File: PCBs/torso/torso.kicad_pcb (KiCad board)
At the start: 4 copper layers, 140 x 81 mm, 84 parts, among them J3 USB_B_Micro, Q1_RLY_CTRL1 Q_NIGBT_CGE, SW1 RESET, U1 TJA1057GT/3J, U2 LM317_TO-220, U3 LM317_TO-220, U4 STM32F303RETx

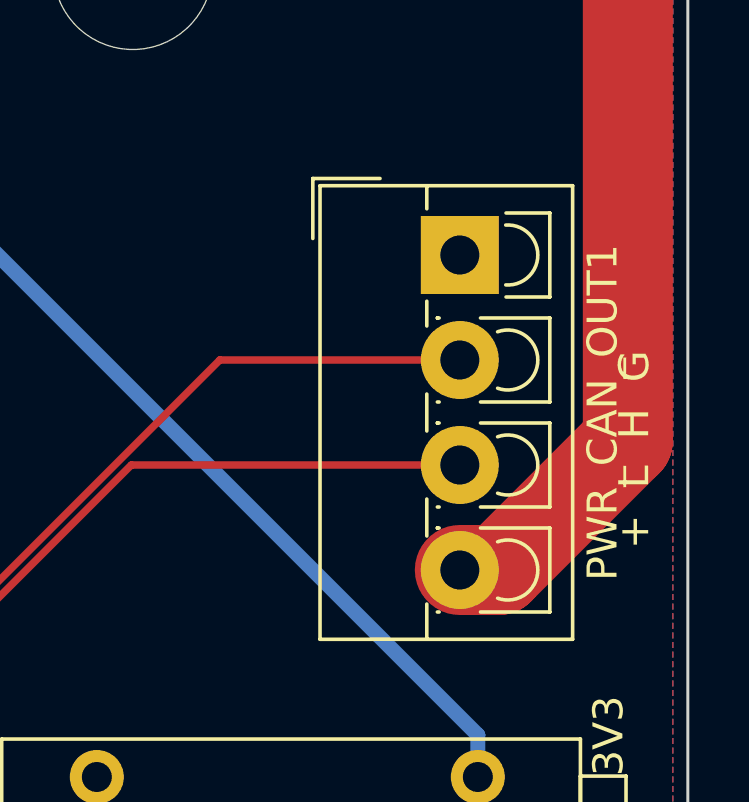
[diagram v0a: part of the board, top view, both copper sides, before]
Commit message: All revisions finished, MK1.1 ready for gerber generation
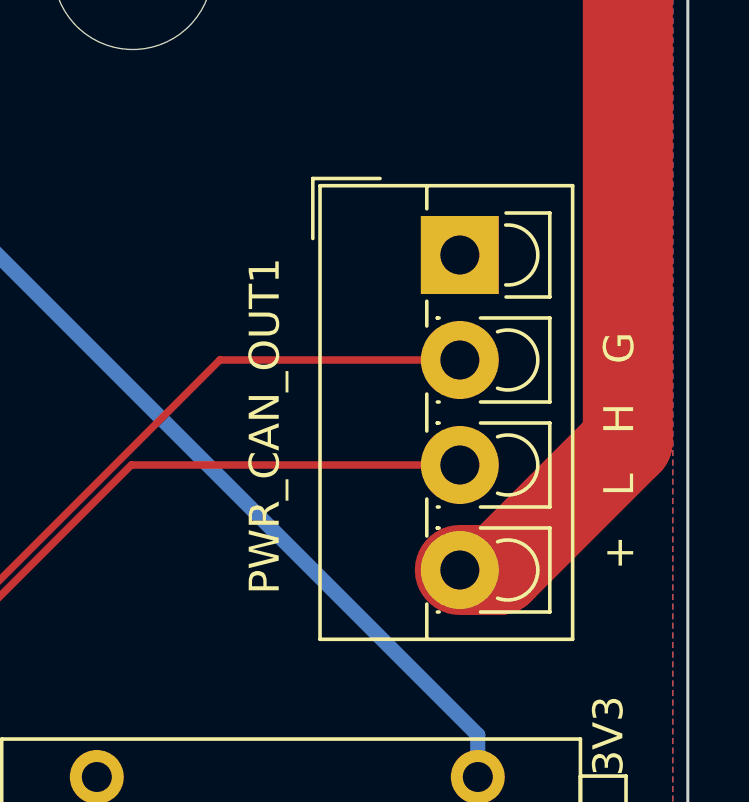
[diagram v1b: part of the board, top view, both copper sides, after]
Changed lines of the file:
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@@
     (property "ki_keywords" "connector")
     (attr through_hole)
-    (fp_text reference "PWR_CAN_OUT1" (at 5.25 -4.76 90) (layer "F.SilkS")
+    (fp_text reference "PWR_CAN_OUT1" (at 5.7 6.5 90) (layer "F.SilkS")
         (effects (font (size 1 1) (thickness 0.15)))
     )
@@
     (effects (font (size 1 1) (thickness 0.1875)) (justify left bottom))
   )
-  (gr_text "+  L  H  G" (at 168.8 50.8 90) (layer "F.SilkS")
+  (gr_text "+   L   H   G" (at 168.3 51.5 90) (layer "F.SilkS")
     (effects (font (size 1 1) (thickness 0.1875)) (justify left bottom))
   )
